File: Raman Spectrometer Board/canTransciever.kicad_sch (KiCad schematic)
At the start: 17 parts, among them SW1 SW_Push, SW2 SW_Push, U6 ATA6561, U7 ATA6561

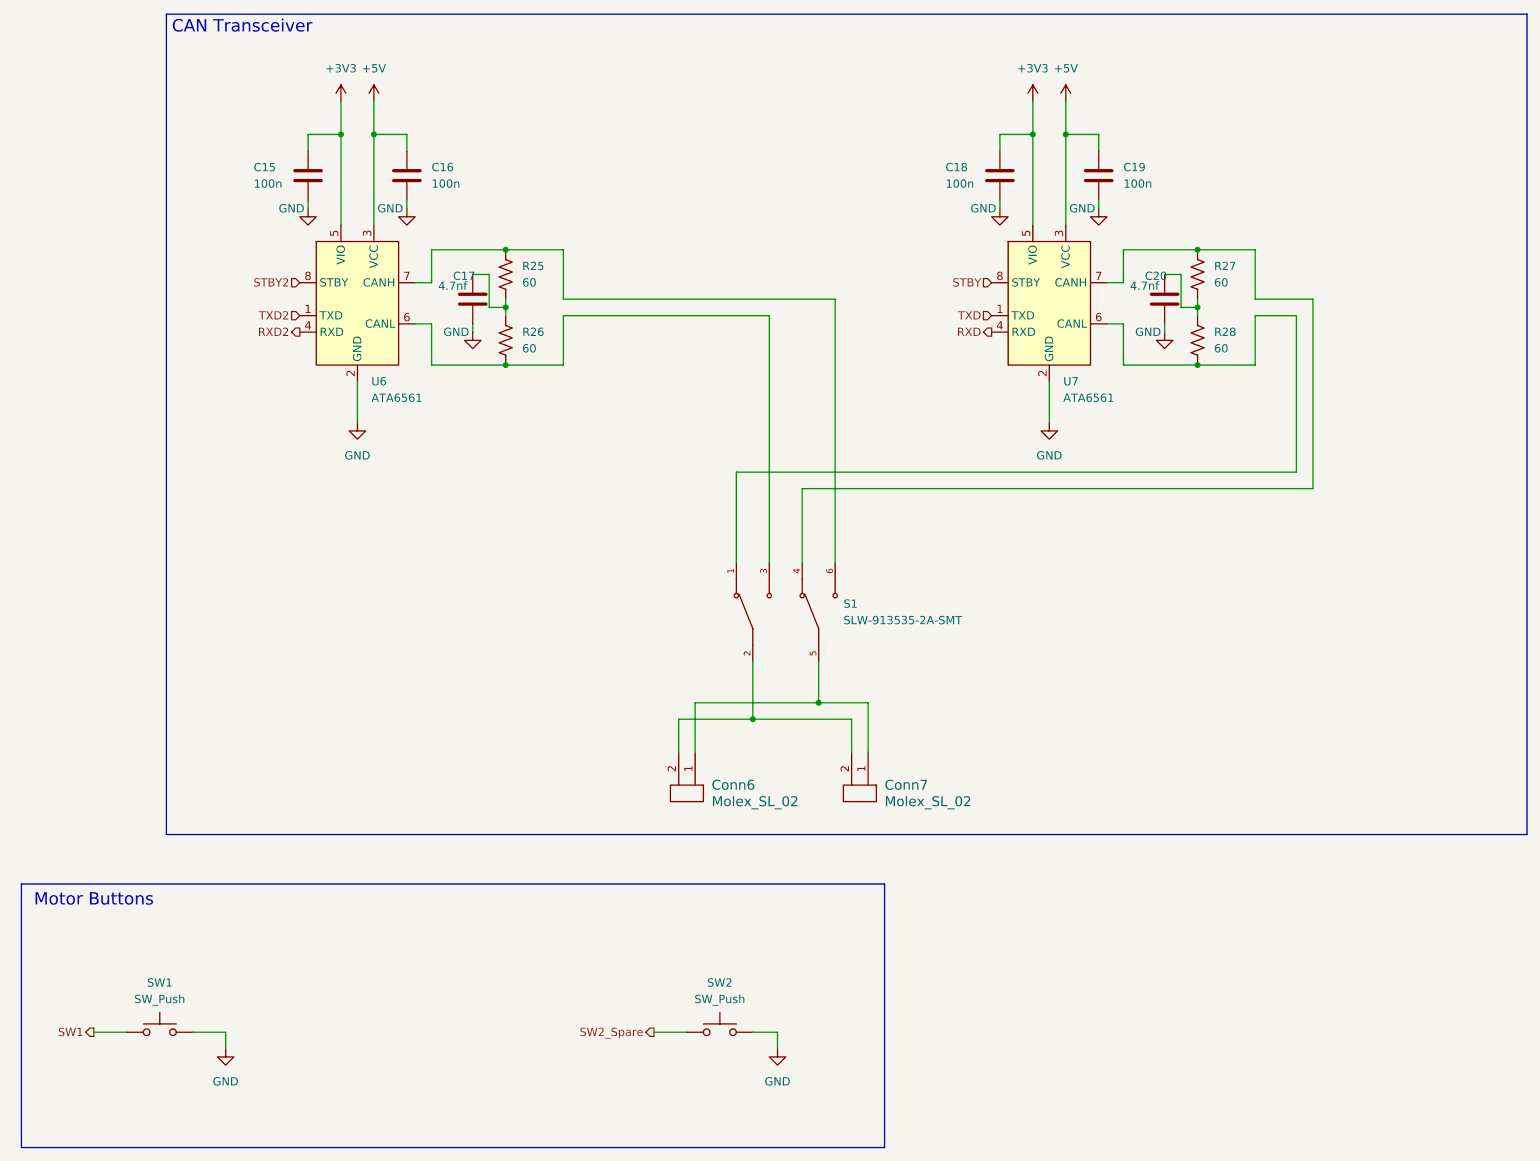
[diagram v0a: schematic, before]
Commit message: Laser switch
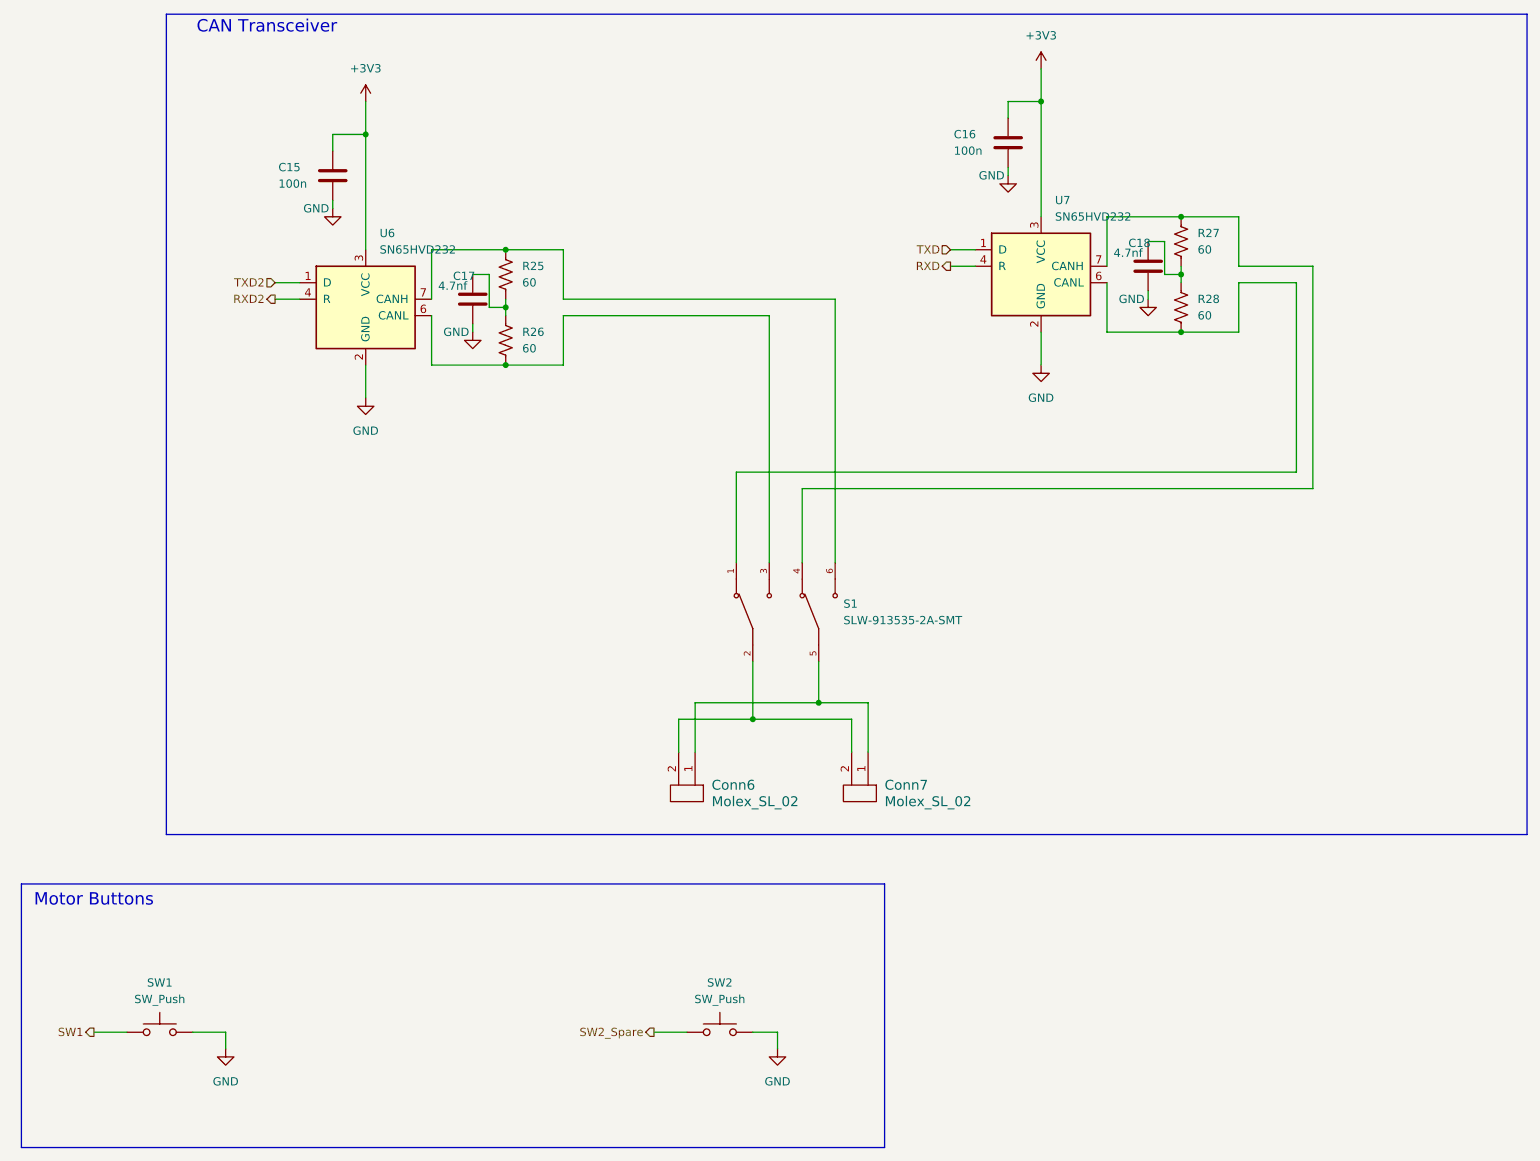
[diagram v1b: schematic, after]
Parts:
- removed C19: 100n, Capacitor_SMD:C_0603_1608Metric_Pad1.08x0.95mm_HandSolder, symbol Device:C
- removed C20: 4.7nf, Capacitor_SMD:C_0603_1608Metric_Pad1.08x0.95mm_HandSolder, symbol Device:C
- removed U6, U7: ATA6561, Package_SO:SOIC-8_3.9x4.9mm_P1.27mm, symbol MRDT_Devices:ATA6561
- added U6, U7: SN65HVD232, Package_SO:SOIC-8_3.9x4.9mm_P1.27mm, symbol Interface_CAN_LIN:SN65HVD232
- C18: value 100n -> 4.7nf
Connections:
- net +5V is gone; now on net +3V3: C16.1
- net +3V3: now also U6.3 (VCC), U7.3 (VCC); no longer C18.1
- net GND: now also U6.2 (GND), U7.2 (GND)
- net RXD: now also U7.4 (R)
- net RXD2: now also U6.4 (R)
- net TXD: now also U7.1 (D)
- net TXD2: now also U6.1 (D)
- net at R28.2, S1.1: now also U7.6 (CANL)
- net at R26.2, S1.3: now also U6.6 (CANL)
- net at R27.1, S1.4: now also U7.7 (CANH)
- net at R25.1, S1.6: now also U6.7 (CANH)
- net at R27.2, R28.1: now also C18.1
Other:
- moved on the sheet: C15
